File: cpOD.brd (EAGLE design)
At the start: 49.5 x 27.9 mm, 31 parts, among them IC1 LM358D, Q1 2N7002

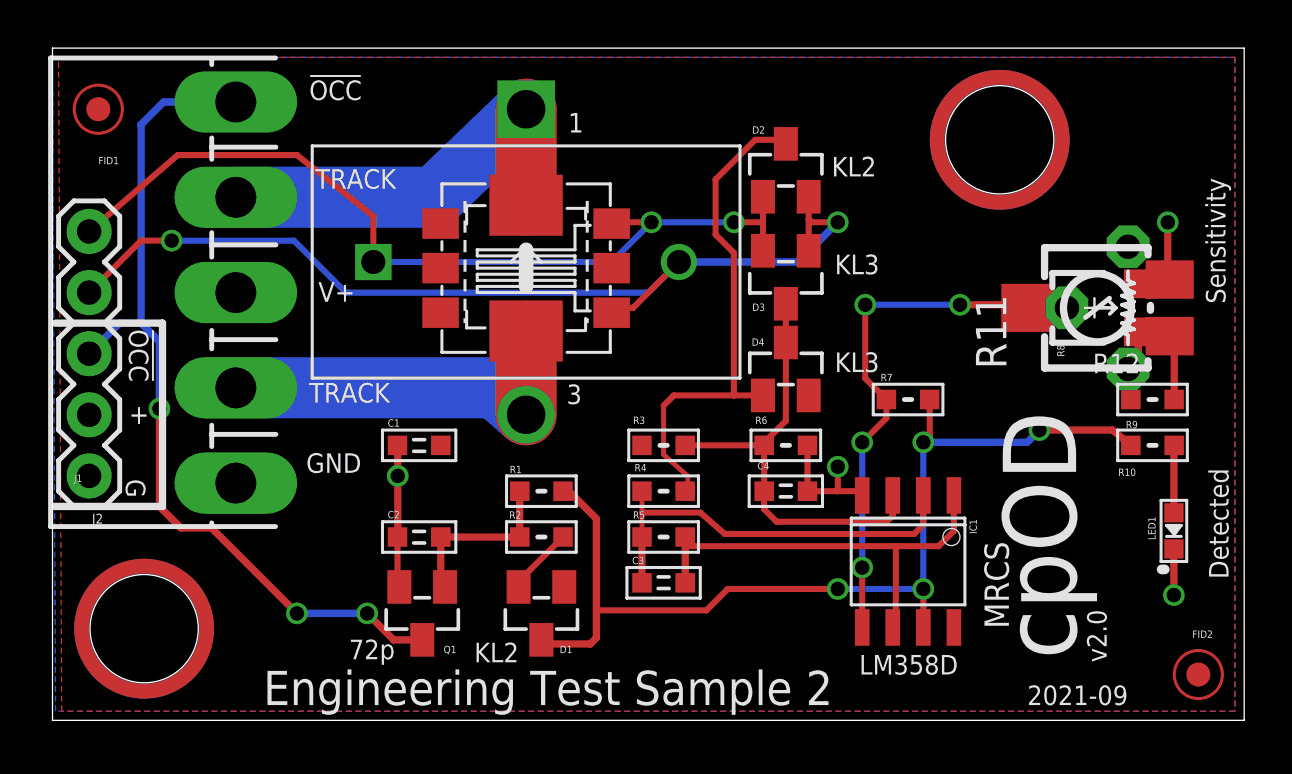
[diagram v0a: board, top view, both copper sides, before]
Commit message: Version 1.1
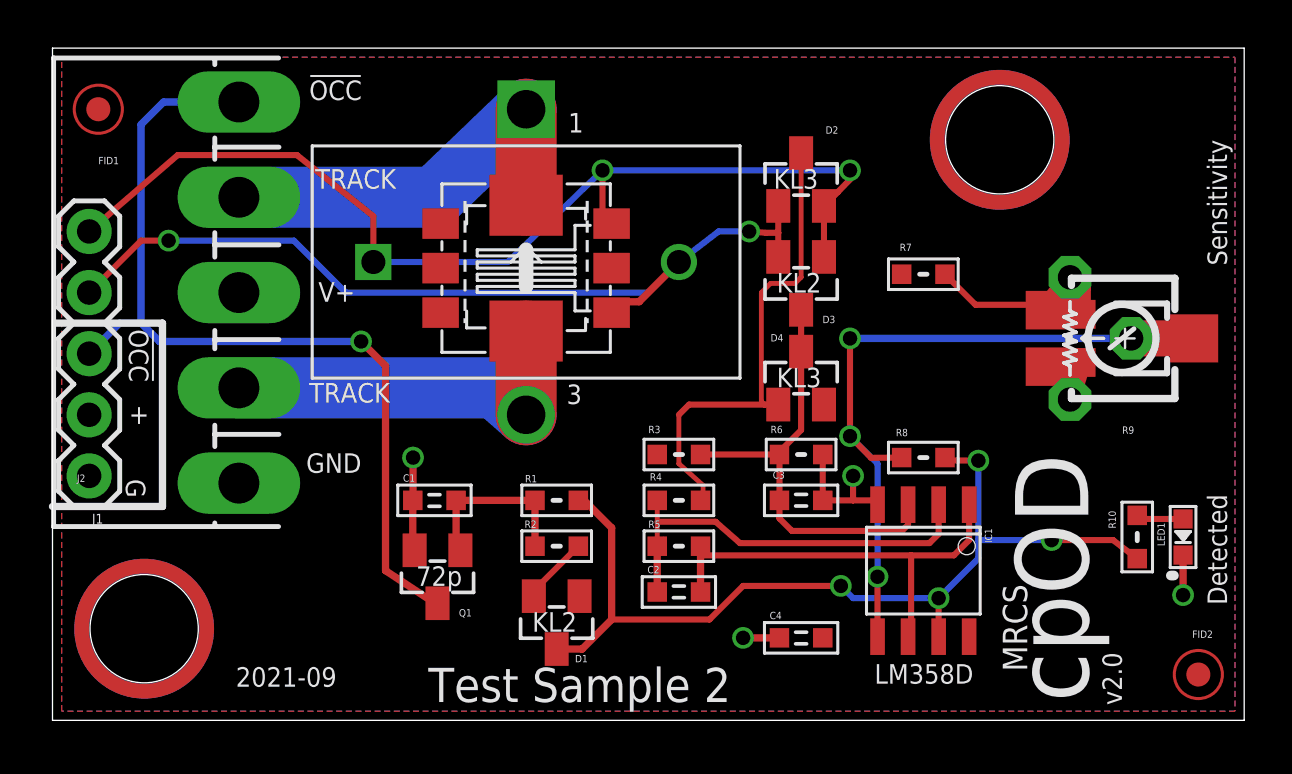
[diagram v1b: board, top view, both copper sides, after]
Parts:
- C1: value 0.1uF -> 1.0uF
- C2: value 1.0uF -> 0.01uF
- C3: value 0.01uF -> 0.1uF
- D2: value BAT54A -> BAT54C
- D3: value BAT54C -> BAT54A
- J1: device SPCoast:KK-156-5 -> SPCoast:1X05
- J2: device SPCoast:1X05 -> SPCoast:KK-156-5
- R10: value 3K3 -> 2k2
- R7: value 1M -> 10K
- R8: value 10K -> 1M; device SPCoast:ST-4 -> SPCoast:0603-RES
- R9: device SPCoast:0603-RES -> SPCoast:ST-4
- moved C2 11.0 mm to (26.0, 5.33), turned to 0 degrees
- moved J2 9.84 mm to (7.75, 17.8)
- moved J1 9.76 mm to (1.52, 10.2)
- moved R8 9.55 mm to (36.2, 10.9), turned to 180 degrees
- moved C3 6.66 mm to (31.1, 9.14)
- moved C4 6.13 mm to (31.1, 3.43), turned to 180 degrees
- moved R7 5.25 mm to (36.2, 18.5)
- moved R10 3.86 mm to (45.1, 7.62), turned to 270 degrees
- moved R9 2.84 mm to (44.5, 15.9), turned to 270 degrees
- moved C1 2.37 mm to (15.9, 9.14)
- moved R12 1.80 mm to (44.6, 15.9), turned to 270 degrees
- moved Q1 1.65 mm to (16.0, 5.97)
- moved R11 1.28 mm to (43.6, 15.9), turned to 270 degrees
- moved R3 0.74 mm to (26.0, 11.0)
- moved R4 0.74 mm to (26.0, 9.14)
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- renumbered U$5 to U$1, U$6 to U$2
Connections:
- net !VOUT: now also J1.3, J2.5; no longer J1.5, J2.3
- net DCC-A: now also J2.2; no longer J1.2
- net DCC-B: now also J2.4; no longer J1.4
- net DETECTED: now also R8.1; no longer R7.1
- net GND: now also C3.2, R9.2; no longer C2.2, R8.2
- net INPUT-A: now also D2.1, D3.2, J1.4; no longer D2.2, D3.1, J2.4
- net INPUT-B: now also D2.2, D3.1, J1.5; no longer D2.1, D3.2, J2.5
- net OCCUPIED: now also C1.1; no longer C2.1
- net SENS+: now also R7.1; no longer R8.1
- net SENSITIVITY: now also R8.2, R9.3; no longer R7.2, R8.3
- net STAGE1+: now also C3.1; no longer C4.1
- net STAGE1-: now also C2.1; no longer C3.1
- net TRIGGERED: now also C2.2; no longer C3.2
- net V+: now also C4.1, J1.2, J2.3, R7.2; no longer C1.1, J1.3, J2.2, R9.2
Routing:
- net INPUT-B: track 36.6 -> 43.6 mm
- net SENSITIVITY: track 24.9 -> 29.7 mm, vias 4 -> 3
- net INPUT-A: track 41.3 -> 37.6 mm
- net SENS+: track 5.80 -> 9.40 mm
- net DETECTED: track 41.9 -> 39.4 mm
- net INPUT-NEGATIVE: track 21.6 -> 20.2 mm
- net !VOUT: track 36.9 -> 37.9 mm, vias 3 -> 1
- net N$11: track 2.81 -> 1.97 mm
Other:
- board text added: "Test Sample 2"
- board text removed: "Engineering Test Sample 2"
